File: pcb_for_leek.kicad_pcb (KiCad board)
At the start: 2 copper layers, 130 x 44.2 mm, 16 parts, among them J1 Conn_01x08_MountingPin, J3 Conn_01x02, SW1 SW_Push, SW10 JS102011SAQN, SW2 SW_Push, SW3 SW_Push, SW4 SW_Push, SW5 SW_Push, SW6 SW_Push, SW7 SW_Push, SW8 SW_Push, SW9 SW_SHDN, U1 SC1176, U2 MAX98357A

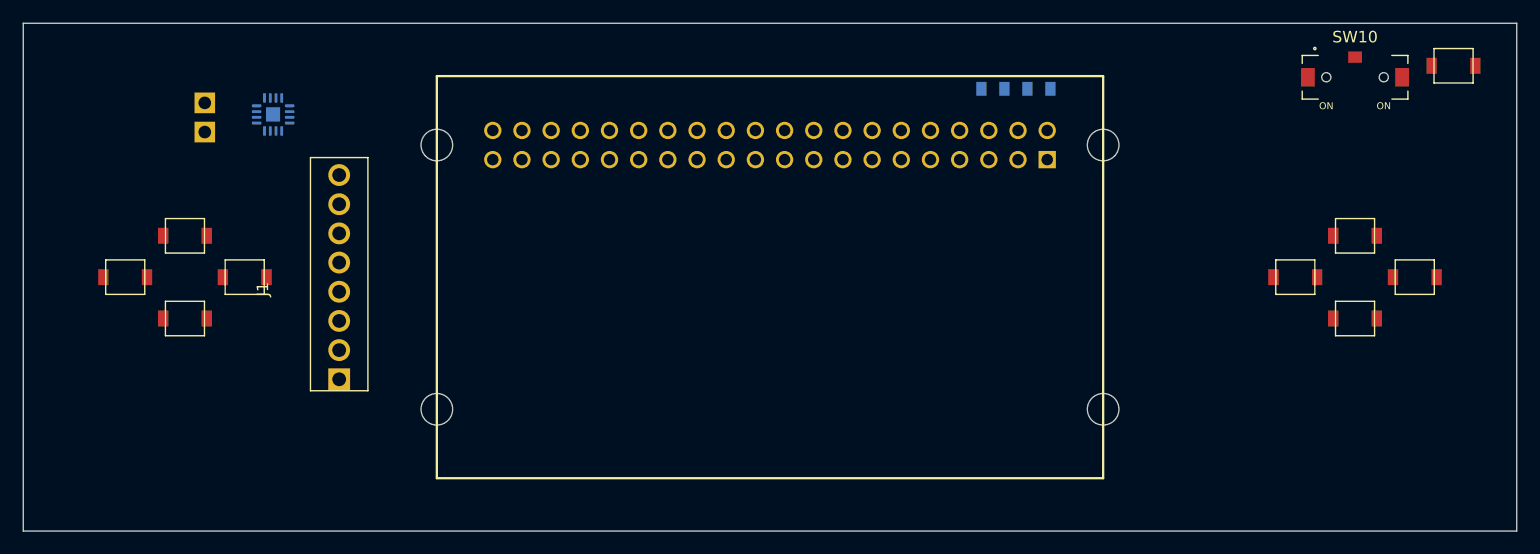
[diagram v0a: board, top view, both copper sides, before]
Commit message: routed pcb
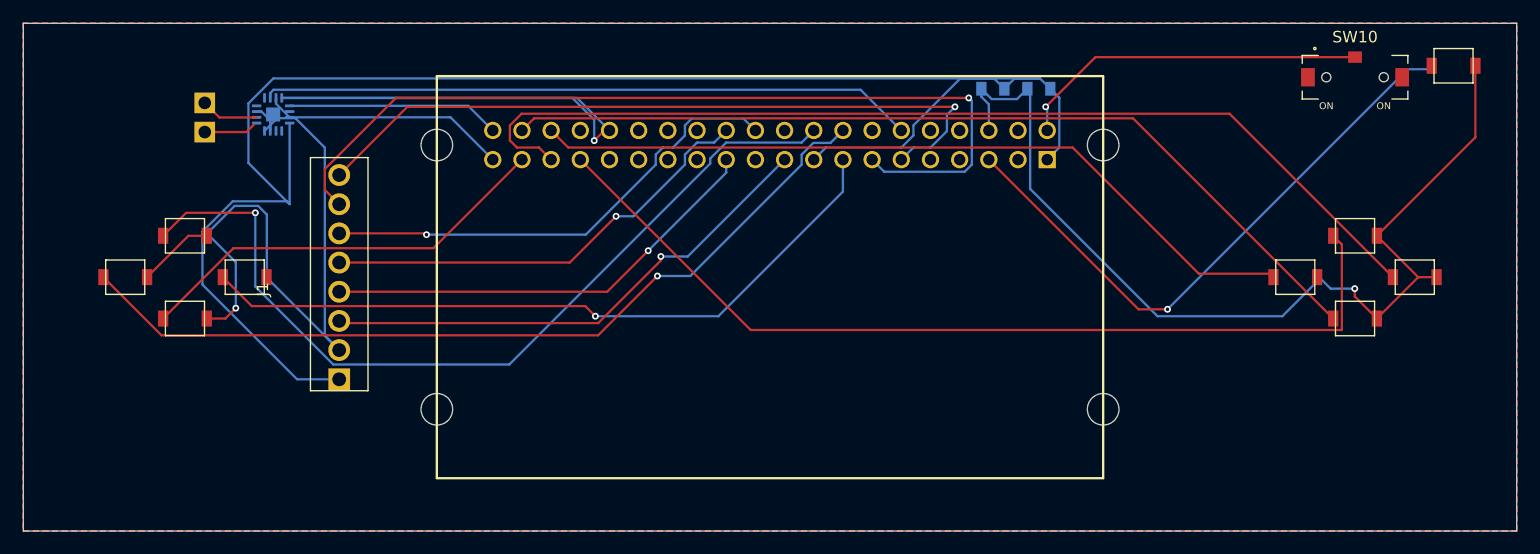
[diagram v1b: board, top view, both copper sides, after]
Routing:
- net GND: track 0.00 -> 172.4 mm, vias 0 -> 2
- net +3.3V: track 0.00 -> 147.7 mm
- net /B: track 0.00 -> 88.8 mm
- net /Y: track 0.00 -> 80.9 mm
- net /A: track 0.00 -> 78.3 mm
- net /GPIO27-13: track 0.00 -> 77.5 mm, vias 0 -> 1
- net /DOWN: track 0.00 -> 75.4 mm, vias 0 -> 1
- net /LEFT: track 0.00 -> 74.4 mm, vias 0 -> 1
- net /X: track 0.00 -> 68.4 mm
- net /GPIO17-11: track 0.00 -> 63.5 mm, vias 0 -> 1
- net /RIGHT: track 0.00 -> 62.7 mm, vias 0 -> 1
- net /GPIO12: track 0.00 -> 61.2 mm, vias 0 -> 1
- net /GPIO18 : track 0.00 -> 56.9 mm
- net /GPIO3: track 0.00 -> 52.7 mm, vias 0 -> 1
- net /MOSI-19: track 0.00 -> 44.9 mm, vias 0 -> 1
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- added copper zone on F.Cu, net (none)
- added copper zone on F.Cu, net GND
